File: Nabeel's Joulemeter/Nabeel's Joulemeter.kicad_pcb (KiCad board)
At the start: 2 copper layers, 89.5 x 84.5 mm, 56 parts, among them J1 430450200, J3 22035035, J4 22035035, J5 430450200, U1 INA181A1QDBVRQ1, U2 PADS131M04QPWRQ1, U3 UA78M05QDCYRG4Q1, U4 MCP6286T-E/OT

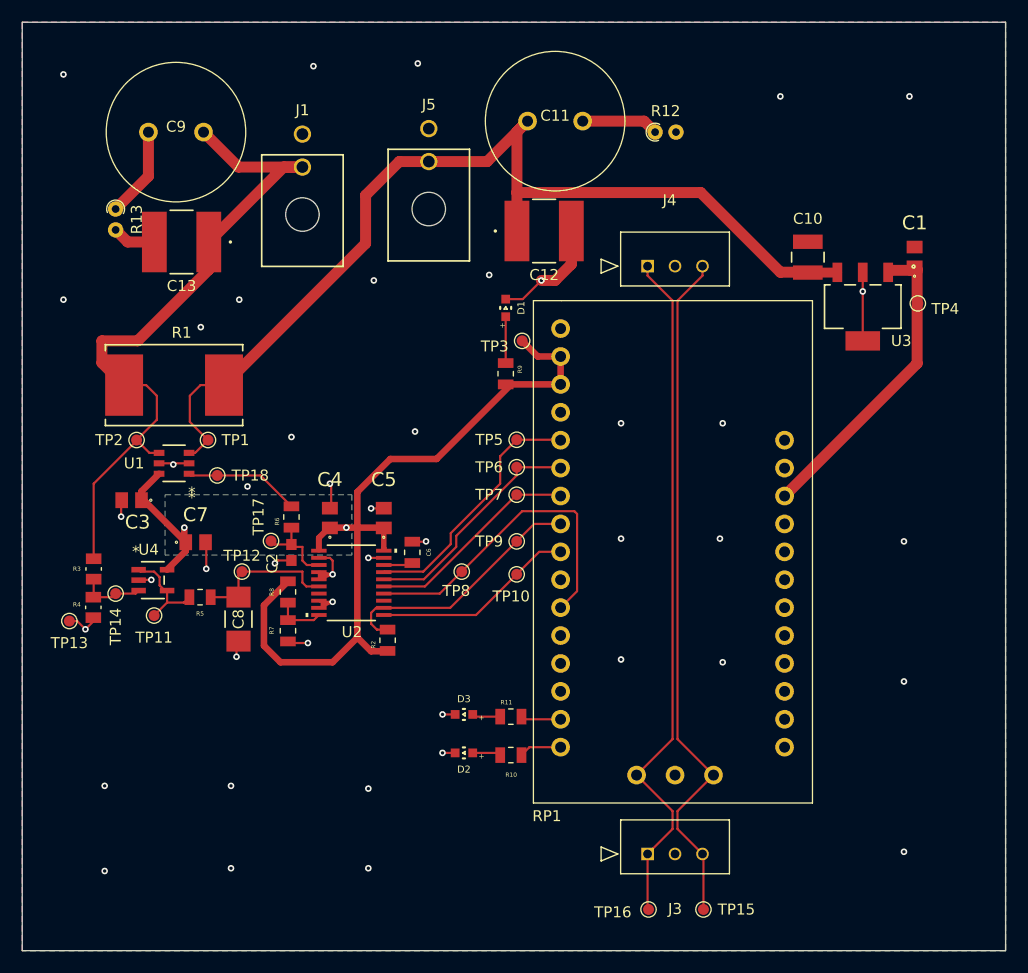
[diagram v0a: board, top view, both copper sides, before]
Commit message: almost final
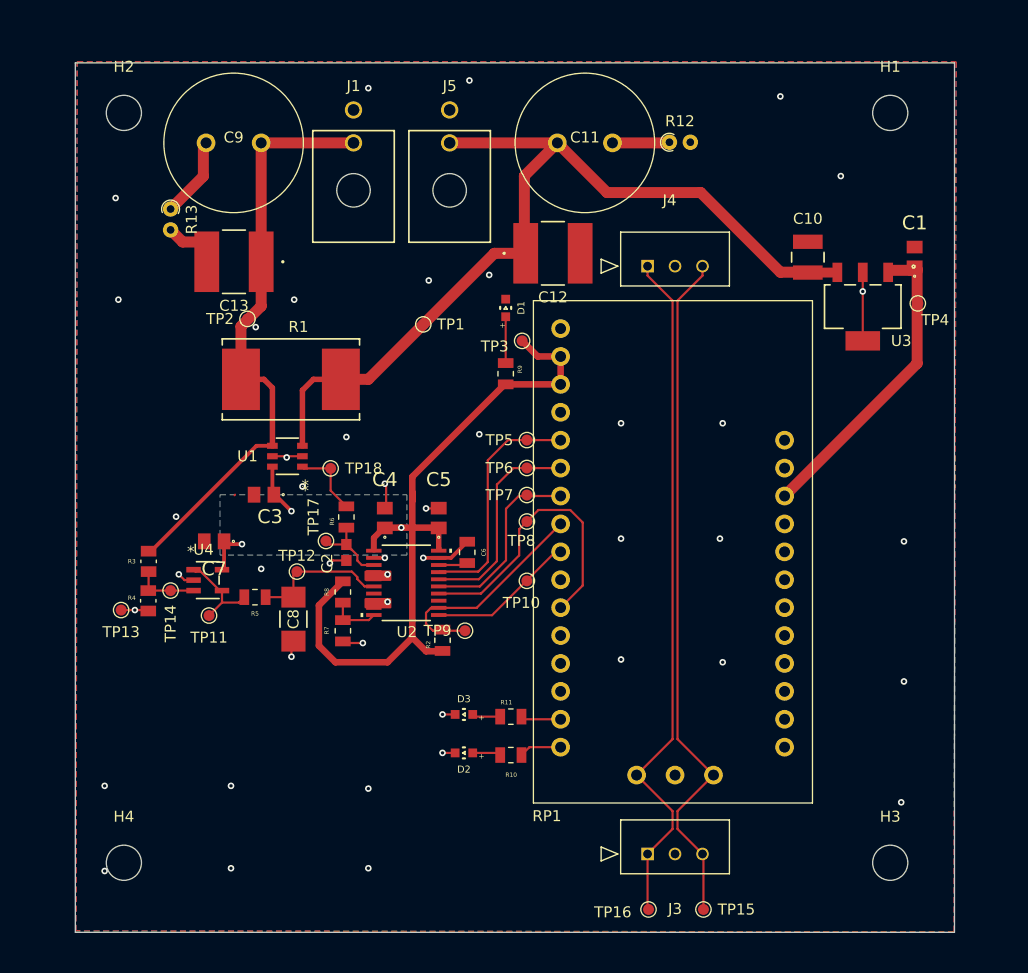
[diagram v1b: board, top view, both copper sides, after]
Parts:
- added H1: MountingHole, MountingHole:MountingHole_3.2mm_M3, F.Cu at (167.5, 65.8)
- added H2: MountingHole, MountingHole:MountingHole_3.2mm_M3, F.Cu at (97.8, 65.8)
- added H3: MountingHole, MountingHole:MountingHole_3.2mm_M3, F.Cu at (167.5, 134.0)
- added H4: MountingHole, MountingHole:MountingHole_3.2mm_M3, F.Cu at (97.8, 134.0)
- moved TP1 22.2 mm to (125.0, 85.0)
- moved TP2 14.9 mm to (109.0, 84.5)
- moved C3 12.1 mm to (110.5, 100.5)
- moved R1 10.6 mm to (113.0, 90.0)
- moved TP18 10.3 mm to (116.6, 98.1)
- moved U1 10.3 mm to (112.6, 97.0)
- moved TP9 9.39 mm to (128.8, 112.9)
- moved TP8 7.48 mm to (134.4, 102.9)
- moved C9 5.34 mm to (107.7, 68.5)
- moved J1 5.14 mm to (118.7, 68.5)
- moved C13 5.10 mm to (107.8, 79.3)
- moved R3 5.05 mm to (100.0, 106.6)
- moved R4 5.04 mm to (100.0, 110.2)
- moved TP14 5.01 mm to (102.0, 109.2)
- moved C2 5.00 mm to (118.0, 105.8)
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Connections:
- C11 pad 3: Net-(C11-Pad2) -> (no net)
- C11 pad 4: +12V -> (no net)
- C9 pad 3: /SHUNT_TO_LOAD -> (no net)
- C9 pad 4: Net-(C9-Pad1) -> (no net)
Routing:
- net GND: track 47.7 -> 33.7 mm, vias 46 -> 45
- net +12V: track 93.1 -> 82.0 mm
- net /SHUNT_TO_LOAD: track 64.6 -> 54.4 mm
- net +3.3V: track 86.0 -> 77.7 mm, vias 2 -> 3
- net /GPIO_RESET: track 18.8 -> 13.8 mm
- net Net-(R6-Pad2): track 10.9 -> 7.06 mm
- net /SCK: track 30.0 -> 26.7 mm
- net /CS: track 23.3 -> 20.4 mm
- net /MISO: track 19.6 -> 17.3 mm
- net /MOSI: track 21.4 -> 19.4 mm
- net Net-(C11-Pad2): track 7.01 -> 5.21 mm
- net /GPIO_CLKIN: track 23.2 -> 21.6 mm
- net Net-(C9-Pad1): track 8.24 -> 7.26 mm
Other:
- board size 89.5 x 84.5 mm -> 80 x 79.1 mm
